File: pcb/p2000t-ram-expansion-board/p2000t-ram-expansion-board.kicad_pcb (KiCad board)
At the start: 2 copper layers, 140 x 70 mm, 21 parts, among them J1 EXPANSION BOARD, J2 POWER, U1 74HC04, U2 CY62256-70PC, U3 74HC00, U4 CY62256-70PC, U5 74HC688, U6 74HC32, U7 74HC173, U8 74LHC157

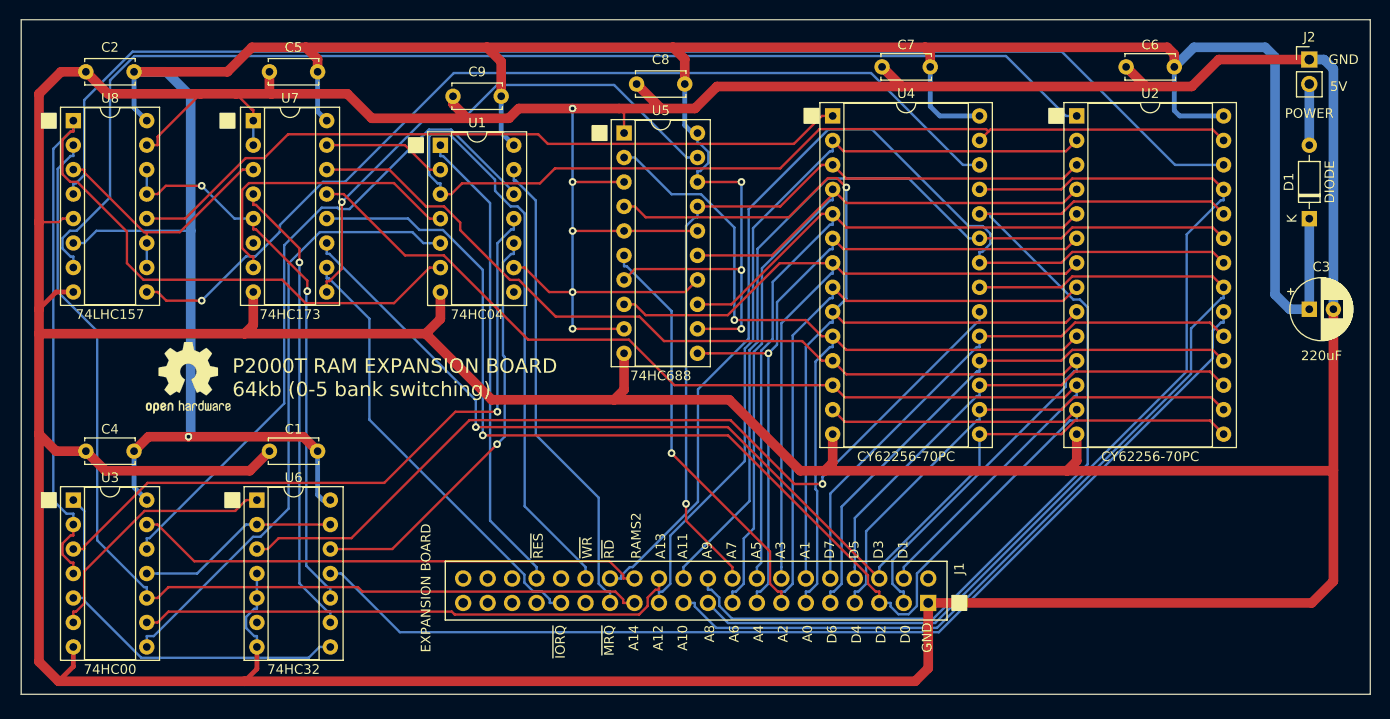
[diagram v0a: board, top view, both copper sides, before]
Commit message: Adding GERBERS
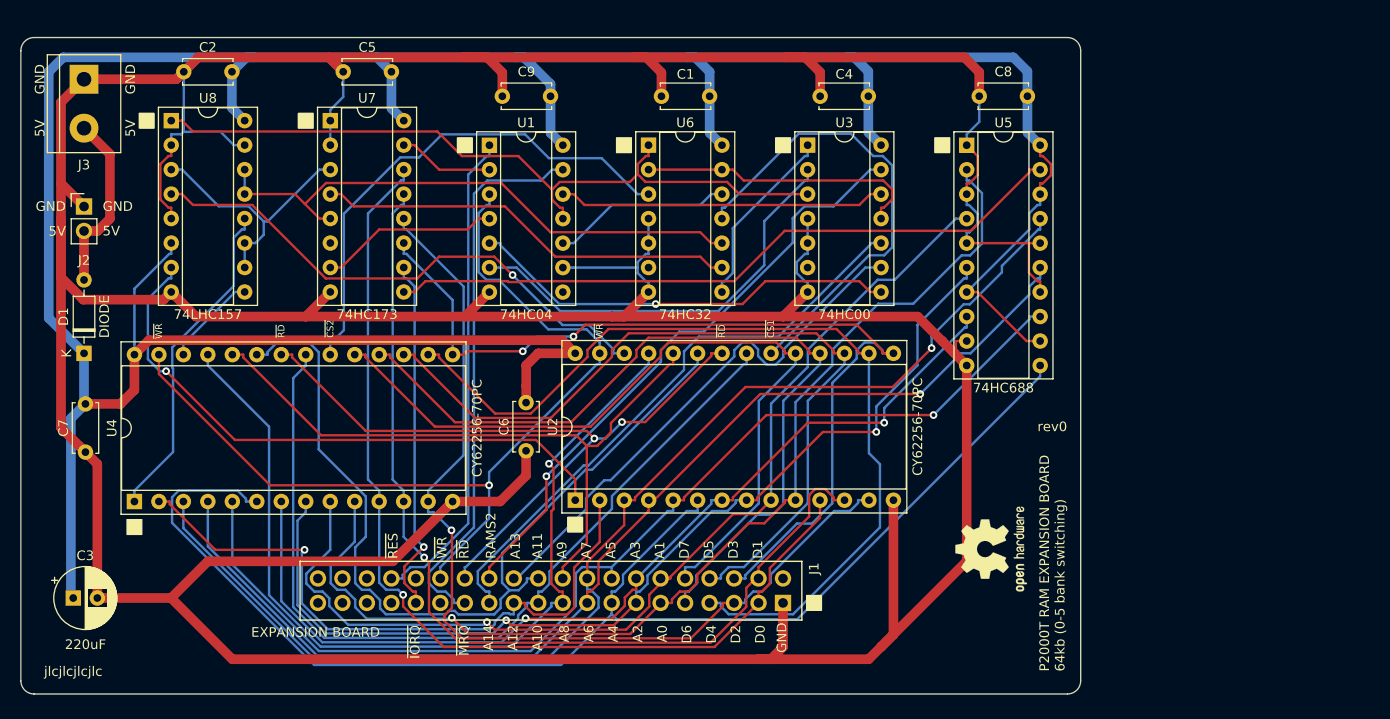
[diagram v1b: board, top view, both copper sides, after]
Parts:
- added J3: TERMINAL, TerminalBlock:TerminalBlock_bornier-2_P5.08mm, F.Cu at (26.5, 26.2)
- moved C3 131.7 mm to (25.4, 80.0)
- moved J2 128.1 mm to (26.5, 39.4)
- moved D1 127.9 mm to (26.5, 54.6)
- moved C7 94.4 mm to (26.7, 59.9), turned to -90 degrees
- moved REF** 85.2 mm to (120.7, 74.9), turned to 90 degrees
- moved U3 84.6 mm to (101.6, 33.0)
- moved C4 84.6 mm to (107.9, 27.9)
- moved U4 82.8 mm to (31.8, 70.0), turned to 90 degrees
- moved C6 75.8 mm to (72.4, 59.7), turned to -90 degrees
- moved U2 65.6 mm to (77.5, 69.9), turned to 90 degrees
- moved C1 54.9 mm to (91.4, 27.9)
- moved U6 54.8 mm to (85.1, 33.0)
- moved C8 35.6 mm to (124.4, 27.9)
- moved U5 35.6 mm to (118.1, 33.0)
- moved J1 15.1 mm to (99.1, 80.5)
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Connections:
- U1 pad 11: Net-(U1-Pad11) -> BR
- U1 pad 6: BR -> Net-(U1-Pad6)
- U3 pad 1: S1 | S2 -> Net-(U3-Pad1)
- U3 pad 2: BR -> Net-(U1-Pad6)
- U3 pad 3: Net-(U1-Pad11) -> BR
- U3 pad 4: BR -> GND
- U3 pad 5: S1 | S2 -> GND
- U3 pad 6: Net-(U3-Pad6) -> unconnected-(U3-Pad6)
- U6 pad 1: Net-(U3-Pad6) -> BR
- U6 pad 8: S1 | S2 -> Net-(U3-Pad1)
- U8 pad 2: A14 -> GND
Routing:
- net GND: track 709.7 -> 577.6 mm, vias 5 -> 0
- net A13_2: track 100.9 -> 9.80 mm, vias 1 -> 0
- net A13_1: track 135.6 -> 56.0 mm, vias 0 -> 1
- net Net-(U1-Pad11): track 71.0 -> 0.00 mm, vias 1 -> 0
- net A14_1: track 126.4 -> 62.4 mm, vias 0 -> 1
- net A4: track 75.1 -> 138.9 mm, vias 1 -> 0
- net ~{CS1}: track 111.3 -> 49.0 mm
- net ~{WR}: track 147.2 -> 96.9 mm, vias 0 -> 1
- net D2: track 144.1 -> 99.5 mm
- net Net-(U1-Pad6): track 0.00 -> 44.3 mm
- net A14: track 103.8 -> 61.2 mm
- net D4: track 52.2 -> 94.4 mm
- net A14_2: track 76.4 -> 34.3 mm
- net A7: track 83.6 -> 124.4 mm
- net S1 | S2: track 40.5 -> 0.00 mm
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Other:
- board size 140 x 70 mm -> 110 x 68.1 mm
- board text added: "jlcjlcjlcjlc"
- board text added: "rev0"
- board text added: "~{CS1}"
- board text added: "~{CS2}"
- board text removed: "9.6mm (socket)"
